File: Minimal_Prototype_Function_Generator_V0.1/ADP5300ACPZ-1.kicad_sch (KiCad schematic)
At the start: 10 parts, among them IC2 ADP5300ACPZ-1-R7

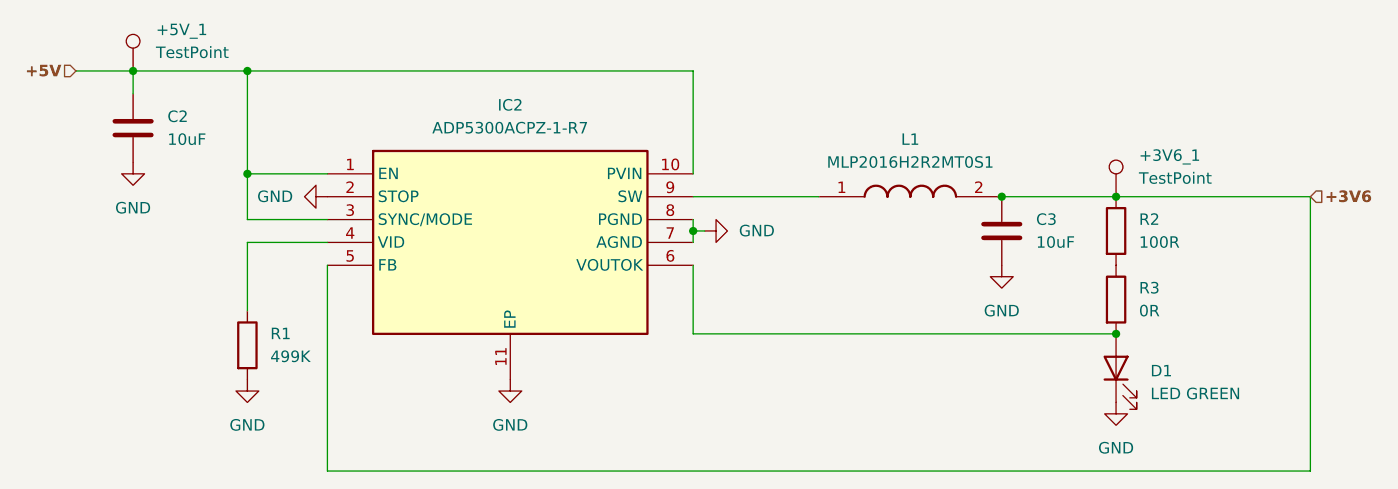
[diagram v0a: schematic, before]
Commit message: new pcb version
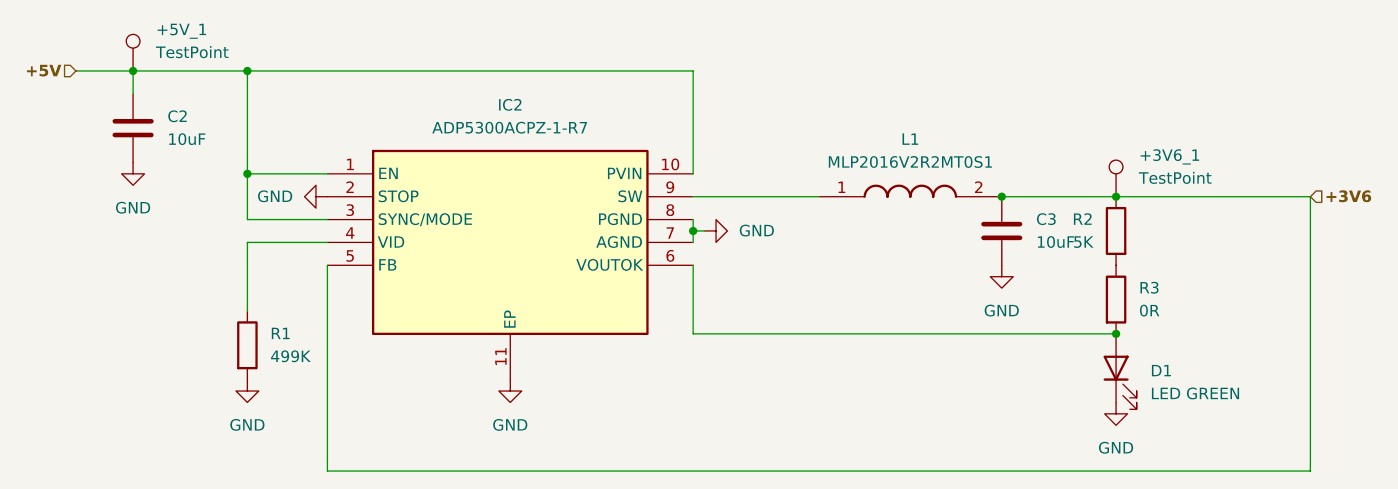
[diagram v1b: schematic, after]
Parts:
- +3V6_1, +5V_1: footprint TestPoint:TestPoint_Loop_D3.80mm_Drill2.5mm -> Insyte_Footprints:Testpoint_hole
- C2, C3: footprint Capacitor_SMD:C_0603_1608Metric -> Insyte_Footprints:C_0603
- D1: footprint LED_SMD:LED_0603_1608Metric -> Insyte_Footprints:CSL1901MW1
- L1: value MLP2016H2R2MT0S1 -> MLP2016V2R2MT0S1; Manufacturer_Part_Number MLP2016H2R2MT0S1 -> MLP2016V2R2MT0S1
- R1, R3: footprint Resistor_SMD:R_0603_1608Metric -> Insyte_Footprints:R_0603
- R2: value 100R -> 5K; footprint Resistor_SMD:R_0603_1608Metric -> Insyte_Footprints:R_0603
